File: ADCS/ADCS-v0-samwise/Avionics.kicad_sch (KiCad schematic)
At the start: 35 parts, among them SW1 KMR231NG LFS, SW2 KMR231NG LFS, U2 RP2350_80QFN, U3 MR25H40MDF, Y1 ABM8-272-T3

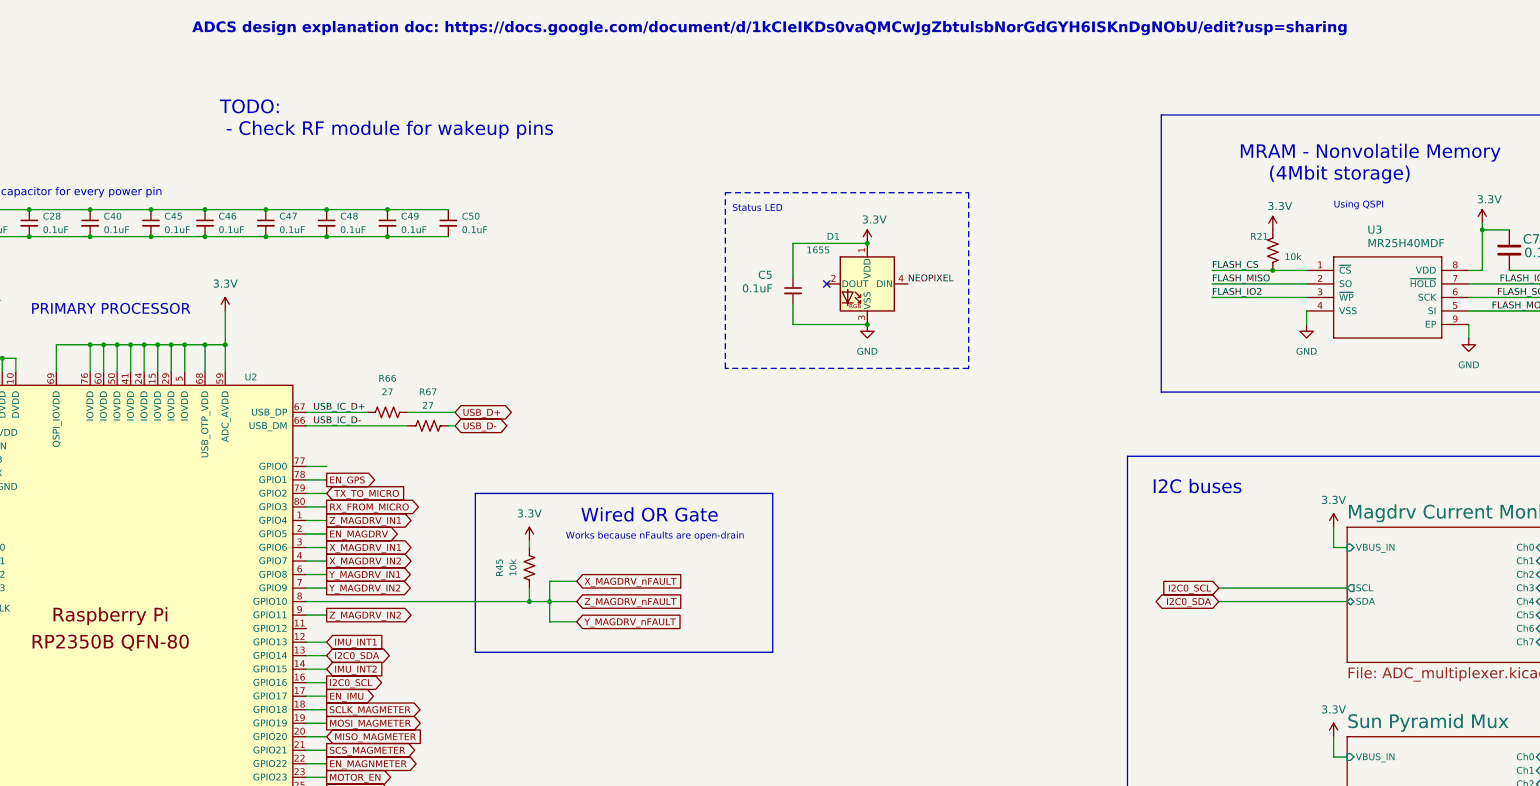
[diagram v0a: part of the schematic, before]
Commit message: incorporated first round of feedbacks
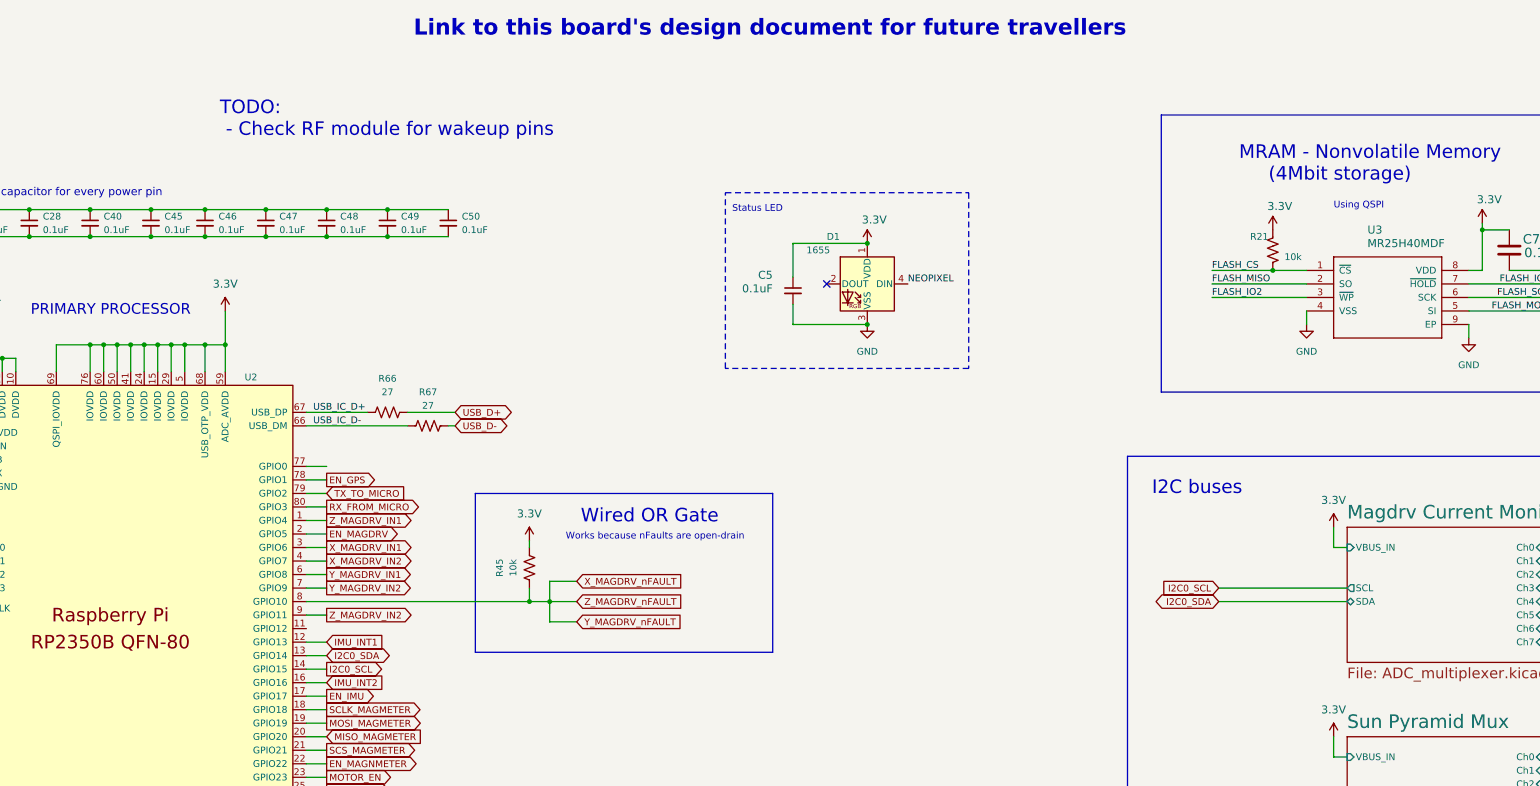
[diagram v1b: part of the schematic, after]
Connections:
- net I2C0_SCL: now also U2.14 (GPIO15); no longer U2.16 (GPIO16)
- net IMU_INT2: now also U2.16 (GPIO16); no longer U2.14 (GPIO15)
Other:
- note added: "Link to this board's design document for future travellers"
- note removed: "ADCS design explanation doc: https://docs.google.com/document/d/1kCIeIKDs0vaQMCwJgZbtulsbNorGdGYH6ISKnDgNObU/edit?usp=sharing"
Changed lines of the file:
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@@
 		)
 	)
-	(text "ADCS design explanation doc: https://docs.google.com/document/d/1kCIeIKDs0vaQMCwJgZbtulsbNorGdGYH6ISKnDgNObU/edit?usp=sharing"
+	(text "Link to this board's design document for future travellers"
 		(exclude_from_sim no)
 		(at 230.632 20.574 0)
 		(effects
 			(font
-				(size 2 2)
+				(size 3 3)
 				(thickness 0.4)
 				(bold yes)
 			)
+			(href "https://docs.google.com/document/d/1kCIeIKDs0vaQMCwJgZbtulsbNorGdGYH6ISKnDgNObU/edit?usp=sharing")
 		)
 	)
@@
 	(global_label "IMU_INT2"
 		(shape input)
-		(at 147.32 140.97 0)
-		(fields_autoplaced yes)
-		(effects
-			(font
-				(size 1.27 1.27)
-			)
-			(justify left)
-		)
-		(property "Intersheetrefs" "${INTERSHEET_REFS}"
-			(at 158.1177 140.97 0)
+		(at 147.32 143.51 0)
+		(fields_autoplaced yes)
+		(effects
+			(font
+				(size 1.27 1.27)
+			)
+			(justify left)
+		)
+		(property "Intersheetrefs" "${INTERSHEET_REFS}"
+			(at 158.1177 143.51 0)
 			(effects
 				(font
@@
 	(global_label "I2C0_SCL"
 		(shape output)
-		(at 147.32 143.51 0)
-		(fields_autoplaced yes)
-		(effects
-			(font
-				(size 1.27 1.27)
-			)
-			(justify left)
-		)
-		(property "Intersheetrefs" "${INTERSHEET_REFS}"
-			(at 158.42 143.51 0)
-			(effects
-				(font
+		(at 147.32 140.97 0)
+		(fields_autoplaced yes)
+		(effects
+			(font
+				(size 1.27 1.27)
+			)
+			(justify left)
+		)
+		(property "Intersheetrefs" "${INTERSHEET_REFS}"
+			(at 158.42 140.97 0)
+			(effects
+				(font
